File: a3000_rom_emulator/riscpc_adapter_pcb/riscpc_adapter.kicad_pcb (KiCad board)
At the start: 2 copper layers, 58.4 x 101.6 mm, 8 parts

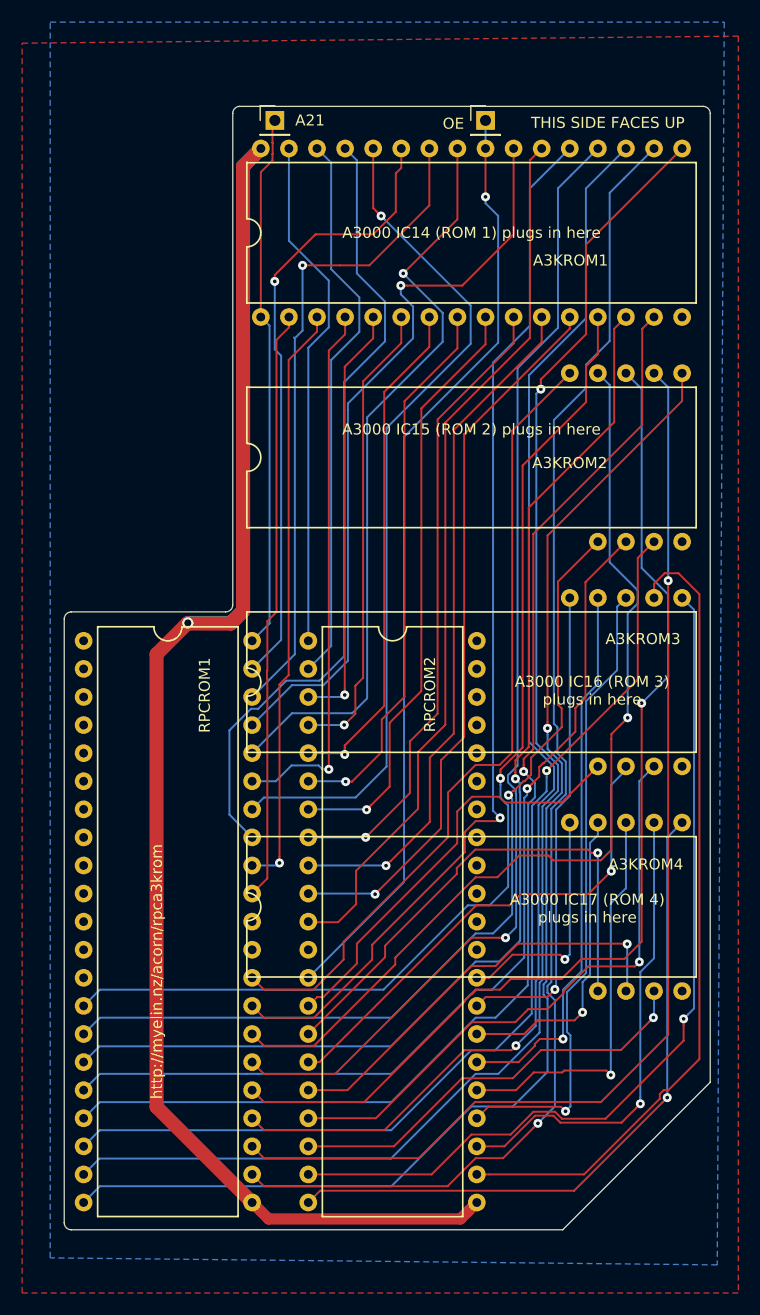
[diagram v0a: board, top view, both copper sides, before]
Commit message: More messing around with traces on riscpc adapter board
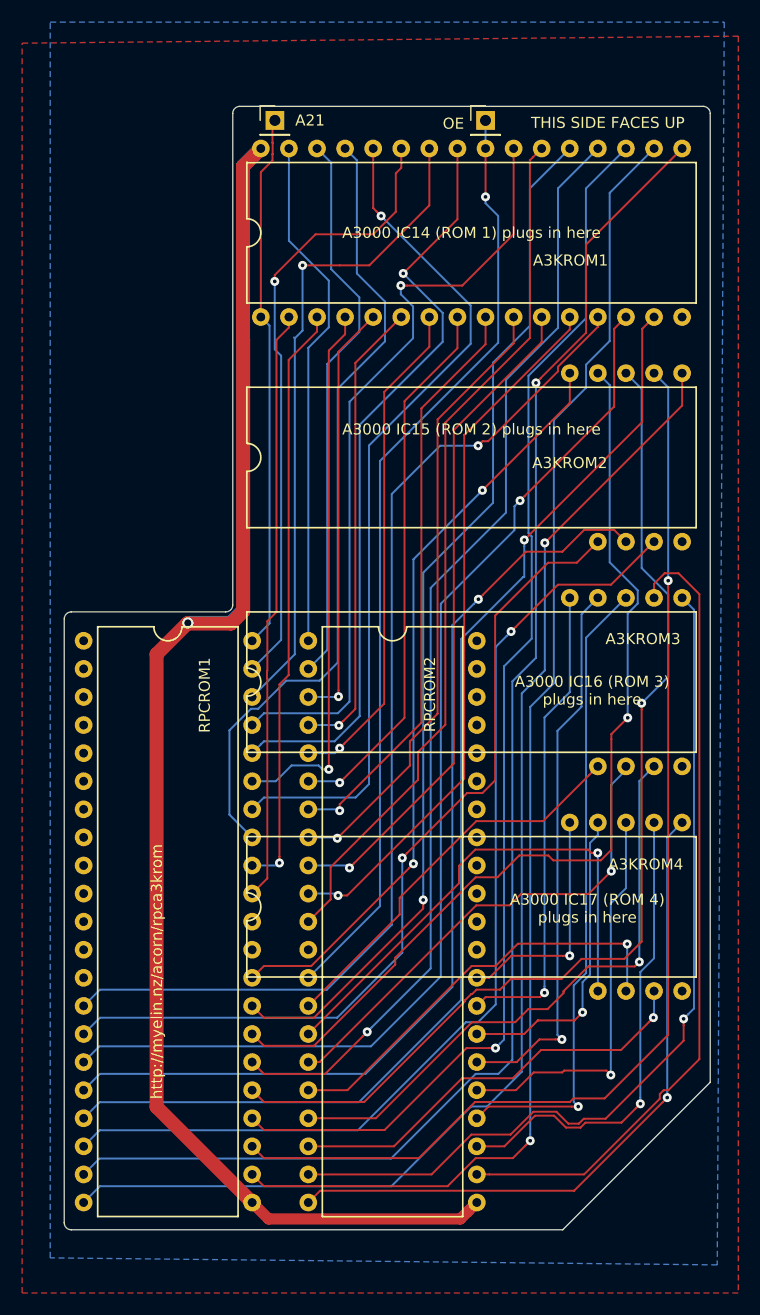
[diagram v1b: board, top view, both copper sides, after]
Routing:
- net D2: track 111.2 -> 107.6 mm
- net D15: track 72.6 -> 69.1 mm, vias 0 -> 2
- net D9: track 86.3 -> 89.6 mm
- net D6: track 103.9 -> 101.0 mm
- net D11: track 116.5 -> 113.7 mm
- net D1: track 104.7 -> 102.1 mm
- net D5: track 114.6 -> 112.0 mm
- net D0: track 98.3 -> 95.9 mm
- net D16: track 38.3 -> 36.0 mm
- net A10: track 67.8 -> 70.0 mm
- net D8: track 80.8 -> 78.7 mm
- net D7: track 95.9 -> 94.2 mm
- net A1: track 62.5 -> 60.8 mm
- net nCS: track 80.3 -> 78.7 mm
- net D3: track 133.5 -> 131.8 mm
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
